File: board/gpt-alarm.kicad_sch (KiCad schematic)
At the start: 12 parts, among them J1 Input, J2 Siren_Out, K1 HK19F-DCxxV-SHC, Q1 AO3400A, Q2 AO3400A

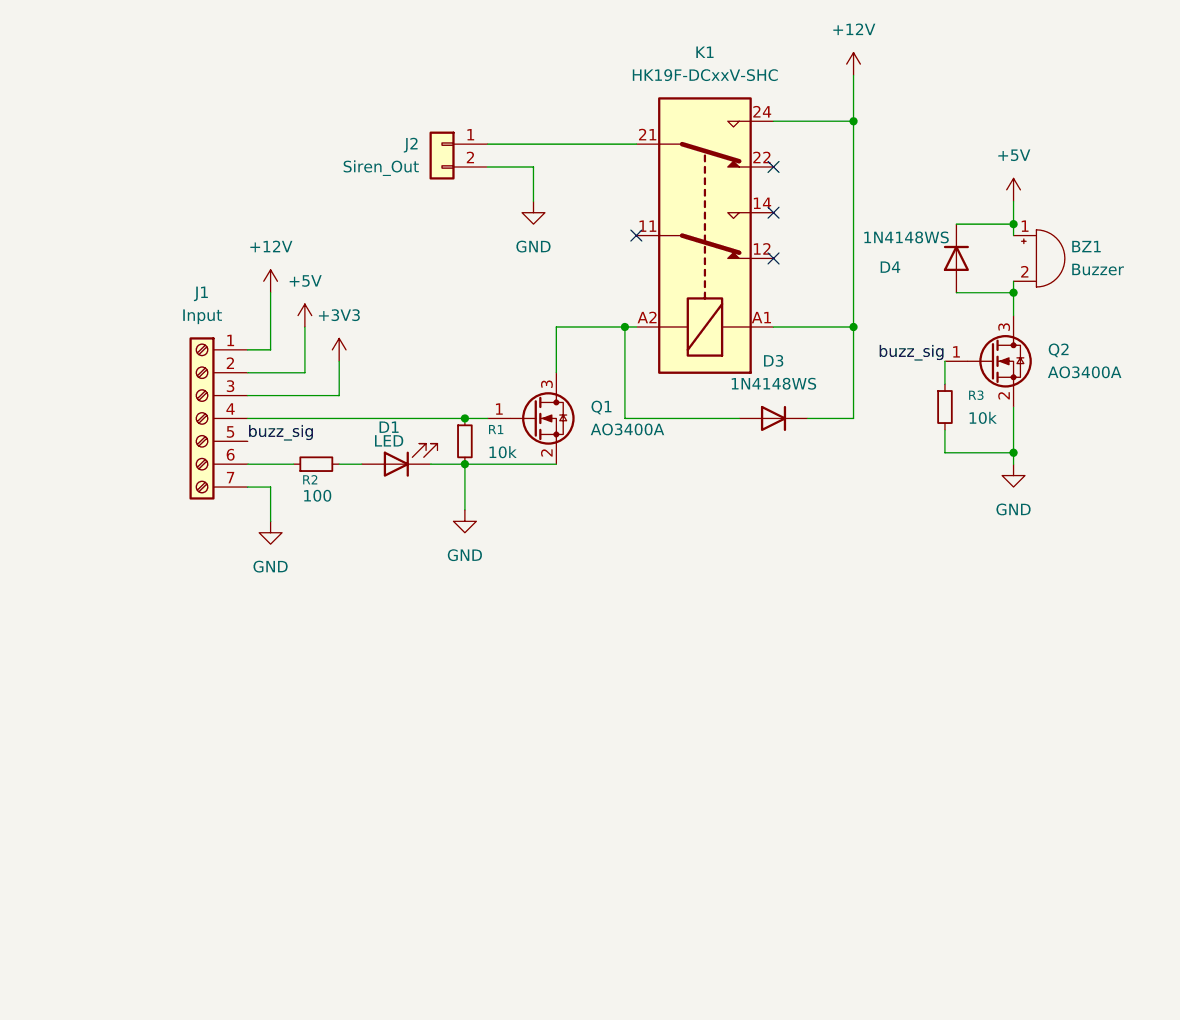
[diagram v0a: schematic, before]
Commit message: feat: pcb layout
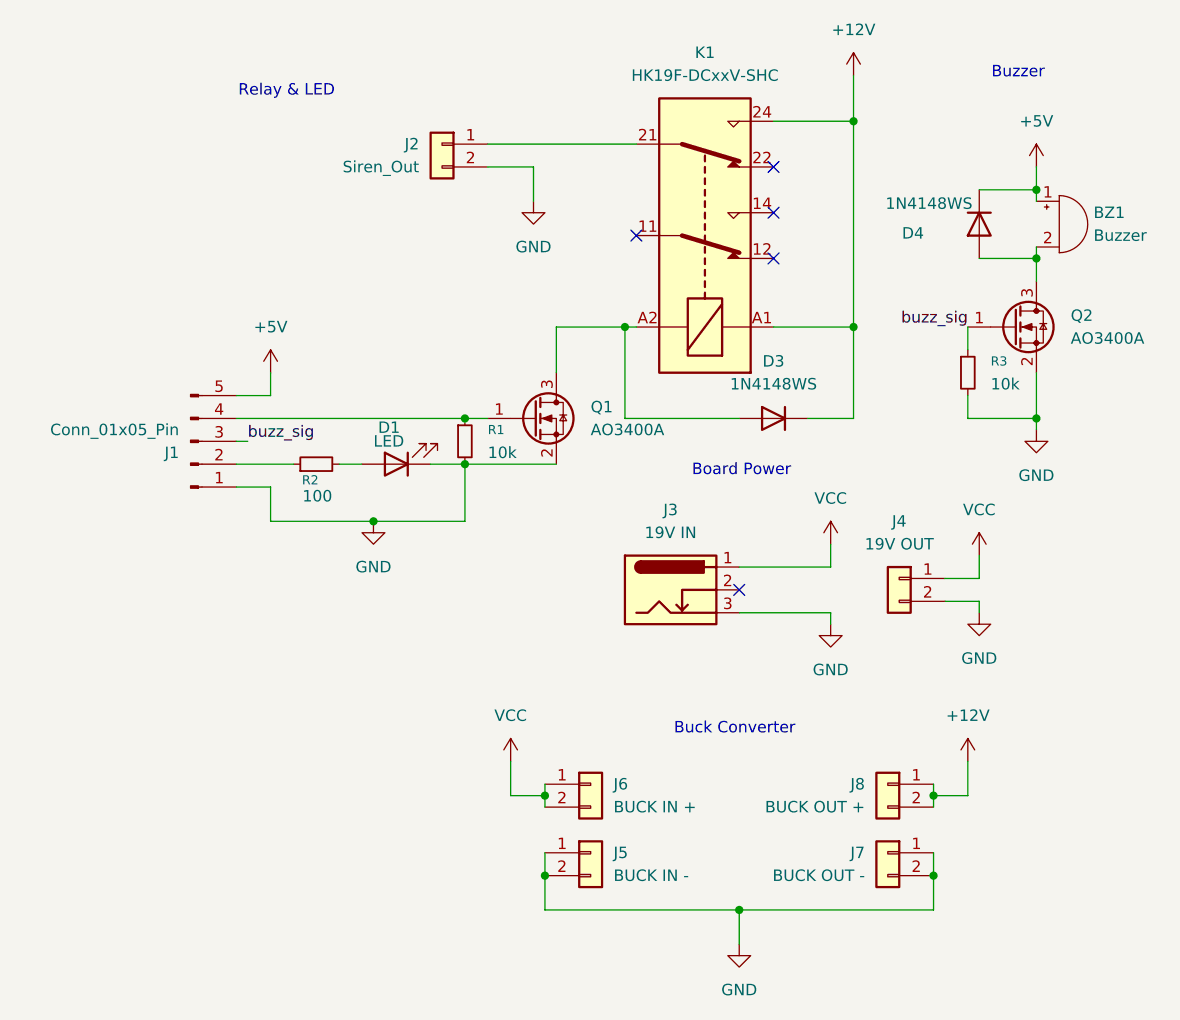
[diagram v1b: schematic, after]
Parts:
- removed J1: Input, TerminalBlock:TerminalBlock_Xinya_XY308-2.54-7P_1x07_P2.54mm_Horizontal, symbol Connector:Screw_Terminal_01x07
- added J1: Conn_01x05_Pin, Connector_PinHeader_2.54mm:PinHeader_1x05_P2.54mm_Horizontal, symbol Connector:Conn_01x05_Pin
- added J3: 19V IN, Connector_BarrelJack:BarrelJack_Horizontal, symbol Connector:Barrel_Jack_Switch_Pin3Ring
- added J4: 19V OUT, TerminalBlock:TerminalBlock_Xinya_XY308-2.54-2P_1x02_P2.54mm_Horizontal, symbol Connector_Generic:Conn_01x02
- added J5: BUCK IN -, Connector_PinHeader_2.54mm:PinHeader_1x02_P2.54mm_Vertical, symbol Connector_Generic:Conn_01x02
- added J6: BUCK IN +, Connector_PinHeader_2.54mm:PinHeader_1x02_P2.54mm_Vertical, symbol Connector_Generic:Conn_01x02
- added J7: BUCK OUT -, Connector_PinHeader_2.54mm:PinHeader_1x02_P2.54mm_Vertical, symbol Connector_Generic:Conn_01x02
- added J8: BUCK OUT +, Connector_PinHeader_2.54mm:PinHeader_1x02_P2.54mm_Vertical, symbol Connector_Generic:Conn_01x02
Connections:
- net +12V: now also J8.1 (Pin_1), J8.2 (Pin_2)
- net +5V: now also J1.5 (Pin_5)
- net GND: now also J1.1 (Pin_1), J3.3, J4.2 (Pin_2), J5.1 (Pin_1), J5.2 (Pin_2), J7.1 (Pin_1), J7.2 (Pin_2)
- net buzz_sig: now also J1.3 (Pin_3)
- net at R2.1: now also J1.2 (Pin_2)
- net at Q1.1 (G), R1.1: now also J1.4 (Pin_4)
- new net VCC: J3.1, J4.1 (Pin_1), J6.1 (Pin_1), J6.2 (Pin_2)
- no-connect marks 4 -> 5
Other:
- note added: "Board Power"
- note added: "Buck Converter"
- note added: "Buzzer"
- note added: "Relay & LED"
- moved on the sheet: BZ1, D4, Q2, R3
